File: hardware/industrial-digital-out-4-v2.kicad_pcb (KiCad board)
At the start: 2 copper layers, 40 x 40 mm, 38 parts, among them P1 CON-SENSOR2, P2 Digital Output, P3 DEBUG, P4 BOOT, Q1 FDN5630, U1 XMC1100, U2 LTV846S, U3 OPA4171AIDR, U4 DRILL, U5 DRILL, U6 DRILL, U7 DRILL

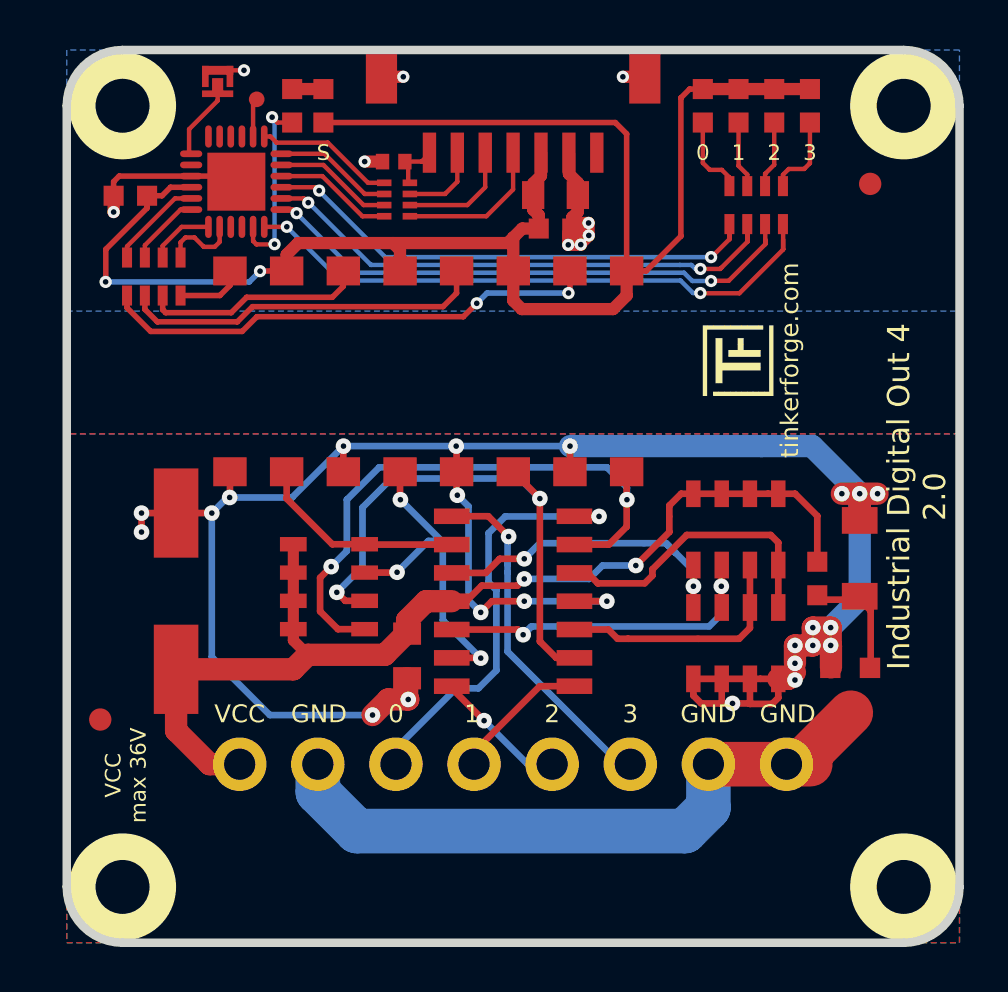
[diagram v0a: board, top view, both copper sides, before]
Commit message: Data Cleanup
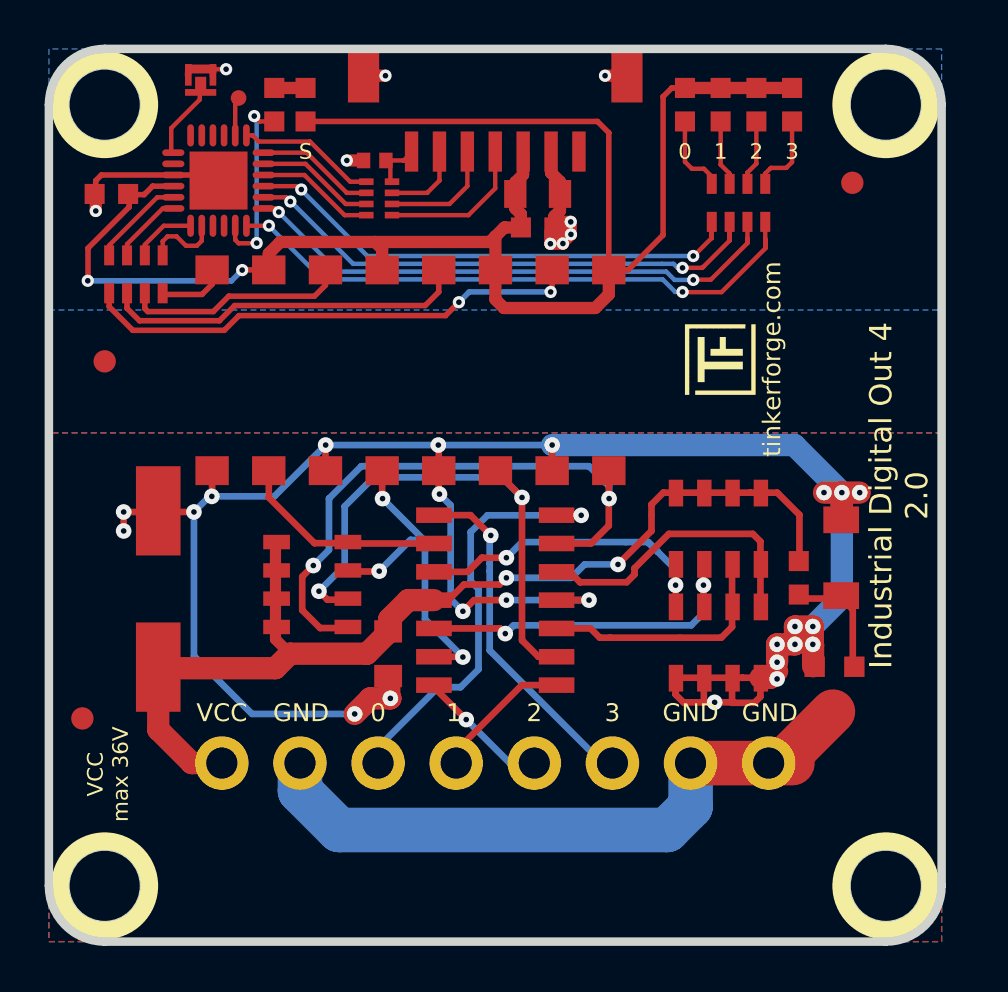
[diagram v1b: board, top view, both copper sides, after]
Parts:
- added Fiducial_Mark: VAL**, kicad-libraries:Fiducial_Mark, F.Cu at (99.5, 52.0)
- moved C2 0.86 mm to (112.2, 65.1)
- moved C6 0.85 mm to (99.8, 44.5)
- moved C4 0.85 mm to (111.6, 43.0)
- moved R1 0.83 mm to (130.6, 61.7)
- moved D1 0.83 mm to (132.5, 60.8)
- moved P3 0.81 mm to (105.5, 40.2)
- moved RP1 0.81 mm to (100.9, 48.1)
- moved C3 0.81 mm to (101.9, 62.2)
- moved Fiducial_Mark 0.80 mm to (98.5, 68.0)
- moved P1 0.80 mm to (117.0, 38.0)
- moved U4 0.80 mm to (134.5, 40.5)
- moved U5 0.80 mm to (134.5, 75.5)
- moved U2 0.80 mm to (113.2, 52.4)
- moved P2 0.80 mm to (117.0, 70.0)
- moved G*** 0.80 mm to (125.5, 53.5)
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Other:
- net class Default removed
- board text added: "Copyright Tinkerforge GmbH 2023. This documentation describes Open Hardware and is licensed under the CERN OHL v. 1.1. You may redistribute and modify this documentation under the terms of the CERN OHL v.1.1. (http://ohwr.org/cernohl). This documentation is distributed WITHOUT ANY EXPRESS OR IMPLIED WARRANTY, INCLUDING OF MERCHANTABILITY, SATISFACTORY QUALITY AND FITNESS FOR A PARTICULAR PURPOSE.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"
- board text removed: "Copyright Tinkerforge GmbH 2018. This documentation describes Open Hardware and is licensed under the CERN OHL v. 1.1. You may redistribute and modify this documentation under the terms of the CERN OHL v.1.1. (http://ohwr.org/cernohl). This documentation is distributed WITHOUT ANY EXPRESS OR IMPLIED WARRANTY, INCLUDING OF MERCHANTABILITY, SATISFACTORY QUALITY AND FITNESS FOR A PARTICULAR PURPOSE.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"
